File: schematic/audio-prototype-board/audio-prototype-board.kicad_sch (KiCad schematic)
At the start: 9 parts, among them IC1 TC1044SCPA, IC2 TC1044SCPA, IC3 TC1044SCPA, IC4 L7805CV, IC5 L7809CV, IC6 L7812CV, J1 163-179PH-EX

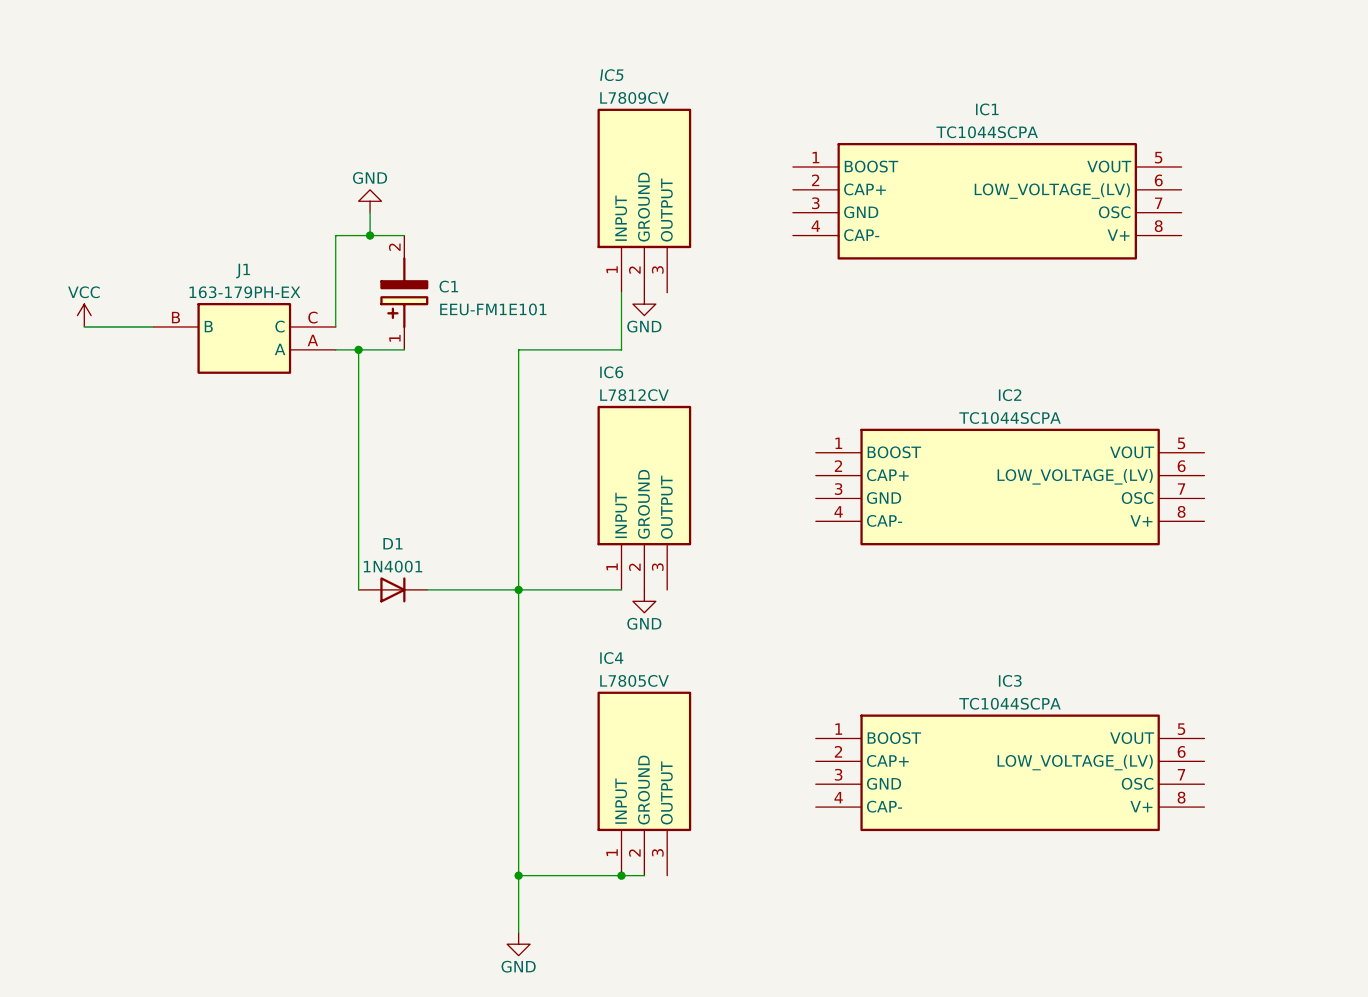
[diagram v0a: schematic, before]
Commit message: Fumbling my way through how to use KiCad.
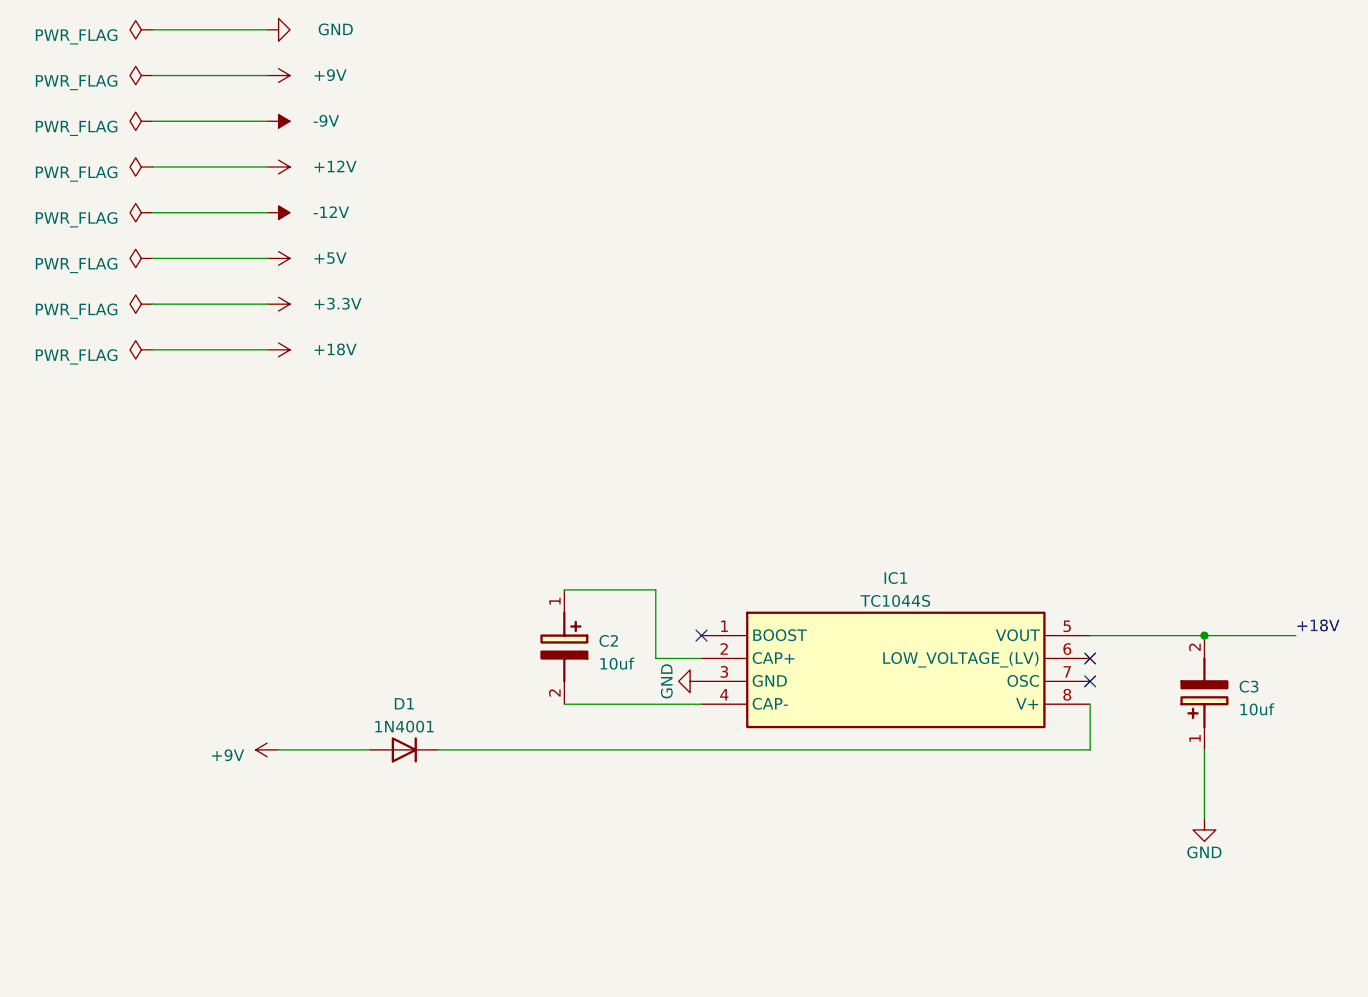
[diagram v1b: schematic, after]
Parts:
- removed C1: EEU-FM1E101, CAPPRD250W55D630H1270, symbol SamacSys_Parts:EEU-FM1E101
- removed IC2, IC3: TC1044SCPA, DIP762W56P254L950H508Q8N, symbol SamacSys_Parts:TC1044SCPA
- removed IC4: L7805CV, TO255P460X1020X2008-3P, symbol SamacSys_Parts:L7805CV
- removed IC5: L7809CV, TO255P460X1020X2008-3P, symbol SamacSys_Parts:L7809CV
- removed IC6: L7812CV, TO255P460X1020X2008-3P, symbol SamacSys_Parts:L7812CV
- removed J1: 163-179PH-EX, 163179PHEX, symbol SamacSys_Parts:163-179PH-EX
- added C2, C3: 10uf, CAPPRD200W50D500H600, symbol SamacSys_Parts:ECE-A1EKS100
- IC1: value TC1044SCPA -> TC1044S
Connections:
- net GND: now also IC1.3 (GND), C3.1 (+); no longer D1.1 (K)
- net at IC1.2 (CAP+): now also C2.1 (+)
- net at IC1.4 (CAP-): now also C2.2 (-)
- net +18V: now reaches IC1.5 (VOUT)
- net +18V: now also C3.2 (-)
- net at IC1.8 (V+): now also D1.1 (K)
- net +9V: now reaches D1.2 (A)
- no-connect marks 0 -> 3
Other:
- moved on the sheet: D1, IC1
